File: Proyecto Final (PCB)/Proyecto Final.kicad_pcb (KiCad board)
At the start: 2 copper layers, 133.5 x 71.2 mm, 55 parts, among them IC1 MC9S08MP16xLC, J1 Input, J10 Relay3, J11 Motor2, J12 Motor4, J13 LCD PINs, J14 Relay2, J15 Relay4, J16 PH_SENSOR, J17 Nivel_L, J18 Nivel_H, J19 Expansion2, J2 Luces_LEDs1, J20 Luces_LEDs2, J3 Expansions5, J4 DHT11_SENSOR, J5 LDR, J6 TDS_SENSOR, J7 Motor1, J8 Motor3, J9 Relay1, K1 FINDER-36.11, K2 FINDER-36.11, K3 FINDER-36.11, K4 FINDER-36.11, Q1 IRF3205, Q2 IRF3205, U1 AP63205WU, U2 MIC4427, U3 TLV2371D, U4 TLV2371D, U5 TLV2371D, U6 PC817, U7 PC817, U8 ULN2803A

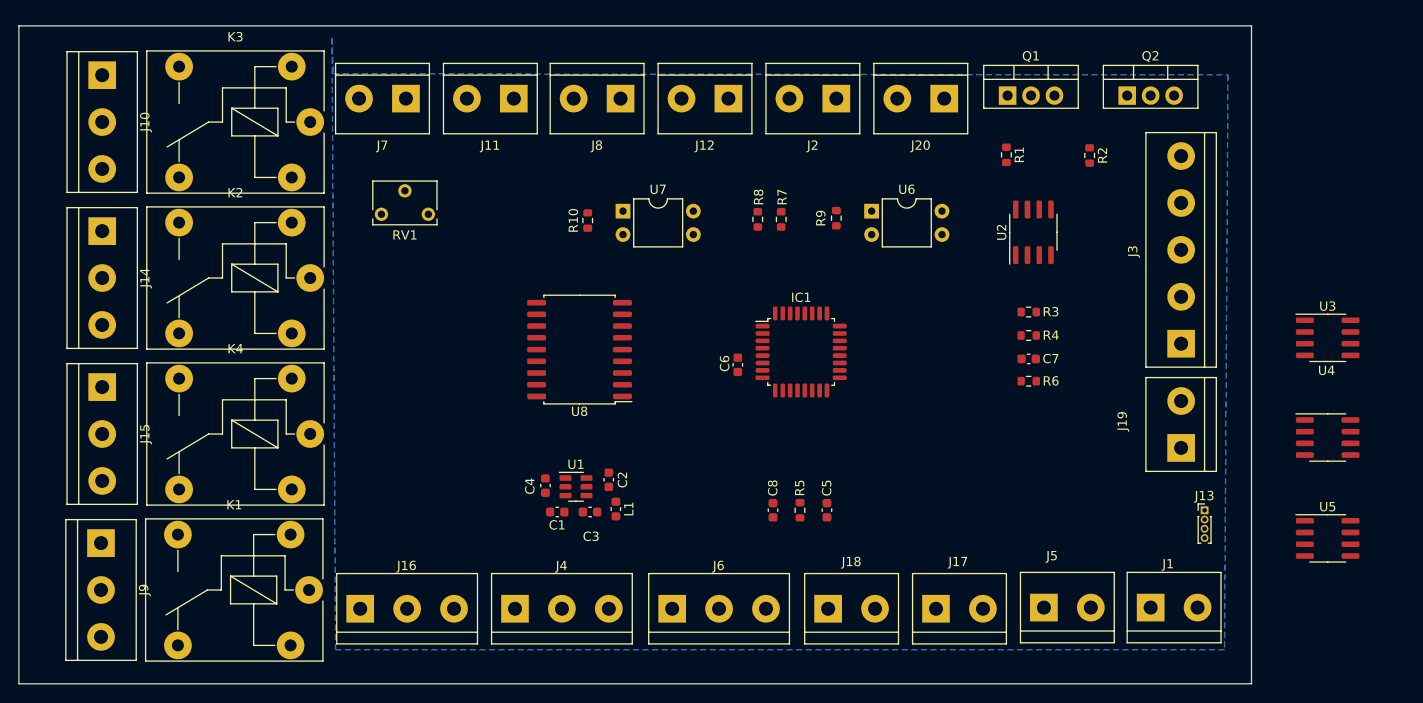
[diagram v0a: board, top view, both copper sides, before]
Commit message: 02/07/2022
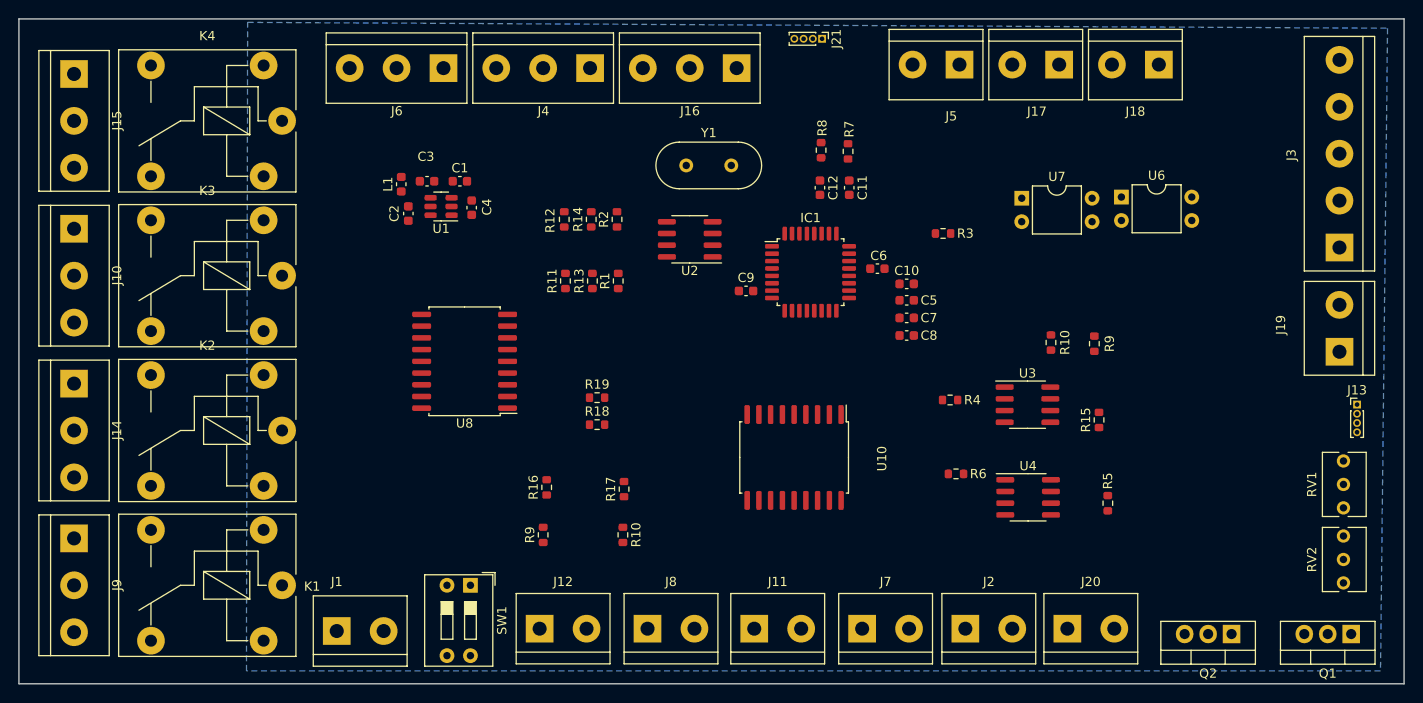
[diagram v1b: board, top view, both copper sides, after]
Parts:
- removed U5: TLV2371D, Package_SO:SOIC-8_3.9x4.9mm_P1.27mm
- added C10: 100nF, Capacitor_SMD:C_0603_1608Metric, F.Cu at (187.3, 91.2)
- added C11: 100nF, Capacitor_SMD:C_0603_1608Metric, F.Cu at (181.1, 80.8)
- added C12: 100nF, Capacitor_SMD:C_0603_1608Metric, F.Cu at (177.9, 80.8)
- added C9: 100nF, Capacitor_SMD:C_0603_1608Metric, F.Cu at (169.9, 91.9)
- added J21: Conn_01x04_Male, Connector_PinHeader_1.00mm:PinHeader_1x04_P1.00mm_Vertical, F.Cu at (178.2, 64.6)
- added R10: 5k, Resistor_SMD:R_0603_1608Metric, F.Cu at (156.6, 118.4)
- added R11: 10k, Resistor_SMD:R_0603_1608Metric, F.Cu at (150.4, 90.9)
- added R12: 10k, Resistor_SMD:R_0603_1608Metric, F.Cu at (150.2, 84.2)
- added R13: 10, Resistor_SMD:R_0603_1608Metric, F.Cu at (153.3, 90.9)
- added R14: 10, Resistor_SMD:R_0603_1608Metric, F.Cu at (153.2, 84.2)
- added R15: 1k, Resistor_SMD:R_0603_1608Metric, F.Cu at (208.2, 105.9)
- added R16: 5k, Resistor_SMD:R_0603_1608Metric, F.Cu at (148.3, 113.2)
- added R17: 5k, Resistor_SMD:R_0603_1608Metric, F.Cu at (156.7, 113.4)
- added R18: 5k, Resistor_SMD:R_0603_1608Metric, F.Cu at (153.8, 106.4)
- added R19: 5k, Resistor_SMD:R_0603_1608Metric, F.Cu at (153.8, 103.5)
- added R9: 5k, Resistor_SMD:R_0603_1608Metric, F.Cu at (148.0, 118.4)
- added RV2: 10k, Potentiometer_THT:Potentiometer_Bourns_3266Y_Vertical, F.Cu at (234.6, 118.5)
- added SW1: SWDIP, Button_Switch_THT:SW_DIP_SPSTx02_Slide_9.78x7.26mm_W7.62mm_P2.54mm, F.Cu at (140.1, 123.8)
- added U10: ULN2803A, Package_SO:SOIC-18W_7.5x11.6mm_P1.27mm, F.Cu at (175.1, 110.0)
- added Y1: Crystal, Crystal:Crystal_HC49-4H_Vertical, F.Cu at (163.4, 78.4)
- R1, R2: value 1k -> 10
- RV1: footprint Potentiometer_THT:Potentiometer_Bourns_3266W_Vertical -> Potentiometer_THT:Potentiometer_Bourns_3266Y_Vertical
- U3, U4: value TLV2371D -> LM358
- moved RV1 107.5 mm to (234.6, 110.4), turned to 90 degrees
- moved J1 88.2 mm to (125.6, 128.8)
- moved J7 75.7 mm to (182.5, 128.5), turned to 0 degrees
- moved J16 71.3 mm to (168.9, 67.8), turned to 180 degrees
- moved Q1 69.2 mm to (235.5, 129.1), turned to 180 degrees
- moved J18 69.0 mm to (214.6, 67.4), turned to 180 degrees
- moved J6 63.6 mm to (137.2, 67.8), turned to 180 degrees
- moved J11 63.0 mm to (170.8, 128.5), turned to 0 degrees
- moved J12 60.9 mm to (147.6, 128.5), turned to 0 degrees
- moved J17 60.4 mm to (203.8, 67.4), turned to 180 degrees
- moved J5 59.5 mm to (193.0, 67.4), turned to 180 degrees
- moved Q2 59.4 mm to (222.5, 129.1), turned to 180 degrees
- moved J4 59.1 mm to (153.0, 67.8), turned to 180 degrees
- moved J2 59.1 mm to (193.7, 128.5), turned to 0 degrees
- moved J20 58.9 mm to (204.7, 128.5), turned to 0 degrees
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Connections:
- net PTC0 renamed PWM_L2
- net PTC1 renamed PWM_L1
- IC1 pad 12: unconnected-(IC1-Pad12) -> Net-(IC1-Pad12)
- IC1 pad 13: SDA_e -> DIP1
- IC1 pad 14: SCL_e -> DIP2
- IC1 pad 15: Motor2 -> Motor3
- IC1 pad 16: Motor3 -> Motor2
- IC1 pad 21: unconnected-(IC1-Pad21) -> +5V
- IC1 pad 22: unconnected-(IC1-Pad22) -> GND
- IC1 pad 23: Motor4 -> Motor1
- IC1 pad 27: unconnected-(IC1-Pad27) -> Net-(IC1-Pad27)
- IC1 pad 28: unconnected-(IC1-Pad28) -> Net-(IC1-Pad28)
- IC1 pad 30: unconnected-(IC1-Pad30) -> Net-(IC1-Pad30)
- IC1 pad 5: Motor1 -> Motor4
- J2 pad 1: +12V -> Net-(Q1-Pad2)
- J2 pad 2: Net-(Q1-Pad2) -> +12V
- J3 pad 3: SDA_e -> SCL
- J3 pad 4: SCL_e -> SDA
- J3 pad 5: ADC_e -> Net-(J3-Pad5)
- RV1 pad 1: GND -> Net-(U6-Pad1)
- RV1 pad 2: GND -> Net-(U6-Pad1)
- RV1 pad 3: Net-(J5-Pad2) -> Net-(J17-Pad2)
- U2 pad 6: +5V -> +12V
- U3 pad 1: unconnected-(U3-Pad1) -> Net-(R4-Pad2)
- U3 pad 5: unconnected-(U3-Pad5) -> Net-(J3-Pad5)
- U3 pad 6: Net-(R4-Pad2) -> Net-(R15-Pad2)
- U3 pad 7: +5V -> Net-(R15-Pad2)
- U3 pad 8: unconnected-(U3-Pad8) -> +5V
- U4 pad 1: unconnected-(U4-Pad1) -> Net-(R6-Pad2)
- U4 pad 2: Net-(R5-Pad2) -> Net-(R6-Pad2)
- U4 pad 3: Net-(J6-Pad3) -> Net-(J16-Pad3)
- U4 pad 5: unconnected-(U4-Pad5) -> Net-(J6-Pad3)
- U4 pad 7: +5V -> Net-(R5-Pad2)
- U4 pad 8: unconnected-(U4-Pad8) -> +5V
- U6 pad 1: Net-(R9-Pad1) -> Net-(U6-Pad1)
- U7 pad 1: Net-(R10-Pad1) -> Net-(U7-Pad1)
- U8 pad 1: Motor4 -> Relay4
- U8 pad 11: M4 -> unconnected-(U8-Pad11)
- U8 pad 12: M3 -> unconnected-(U8-Pad12)
- U8 pad 13: M2 -> unconnected-(U8-Pad13)
- U8 pad 14: M1 -> unconnected-(U8-Pad14)
- U8 pad 2: Motor3 -> Relay3
- U8 pad 3: Motor2 -> Relay2
- U8 pad 4: Motor1 -> Relay1
- U8 pad 5: Relay4 -> unconnected-(U8-Pad5)
- U8 pad 6: Relay3 -> unconnected-(U8-Pad6)
- U8 pad 7: Relay2 -> unconnected-(U8-Pad7)
- U8 pad 8: Relay1 -> unconnected-(U8-Pad8)
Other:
- board size 133.5 x 71.2 mm -> 150 x 72 mm
